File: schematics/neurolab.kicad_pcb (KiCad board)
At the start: 2 copper layers, 127 x 53.6 mm, 159 parts, among them J1 GS3, J10 GS3, J12 GS3, J13 GS3, J14 GS3, J15 GS3, J16 Channel, J17 External, J18 USB_OTG, J19 GS3, J2 GS3, J24 GS2, J3 GS3, J32 Bluetooth, J33 Reset Select, J34 GS2, J4 GS2, J5 GS2, J6 GS3, J7 GS3, J8 PowerOut, J9 GS3, Q1 2N7002, U1 ADP1720ARMZ-5, U10 OPA2111KP, U11 AD8422ARMZ, U12 OP4117, U13 OPA2111KP, U14 AD8422ARMZ, U15 OP4117, U16 AD7173, U17 ADR445BR, U18 Arduino, U2 ADP1720ARMZ-3.3, U3 AD8475, U4 AD8475, U5 MAX7480ESA+, U6 MAX7480ESA+, U7 MAX7480ESA+, U8 MAX7480ESA+, U9 TLC555CD, Y1 FA-20H

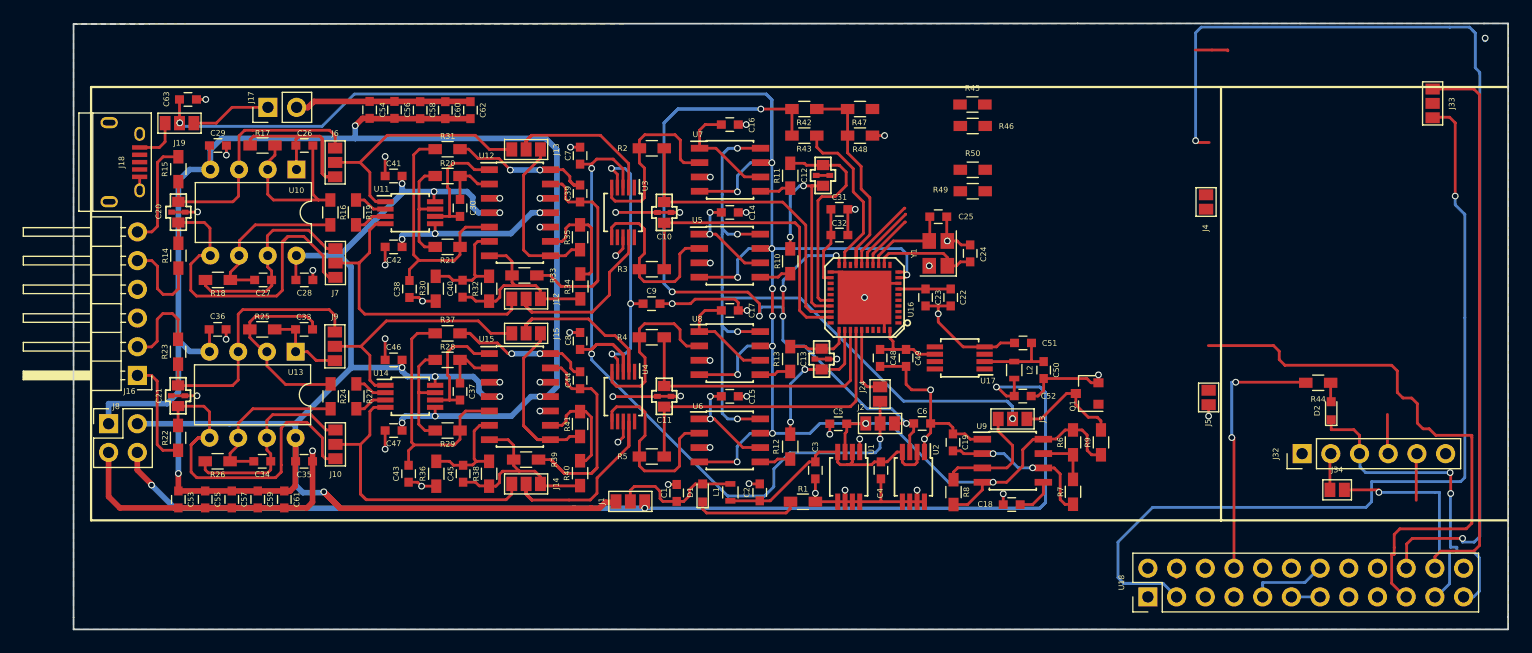
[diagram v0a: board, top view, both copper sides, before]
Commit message: optimize: final routing
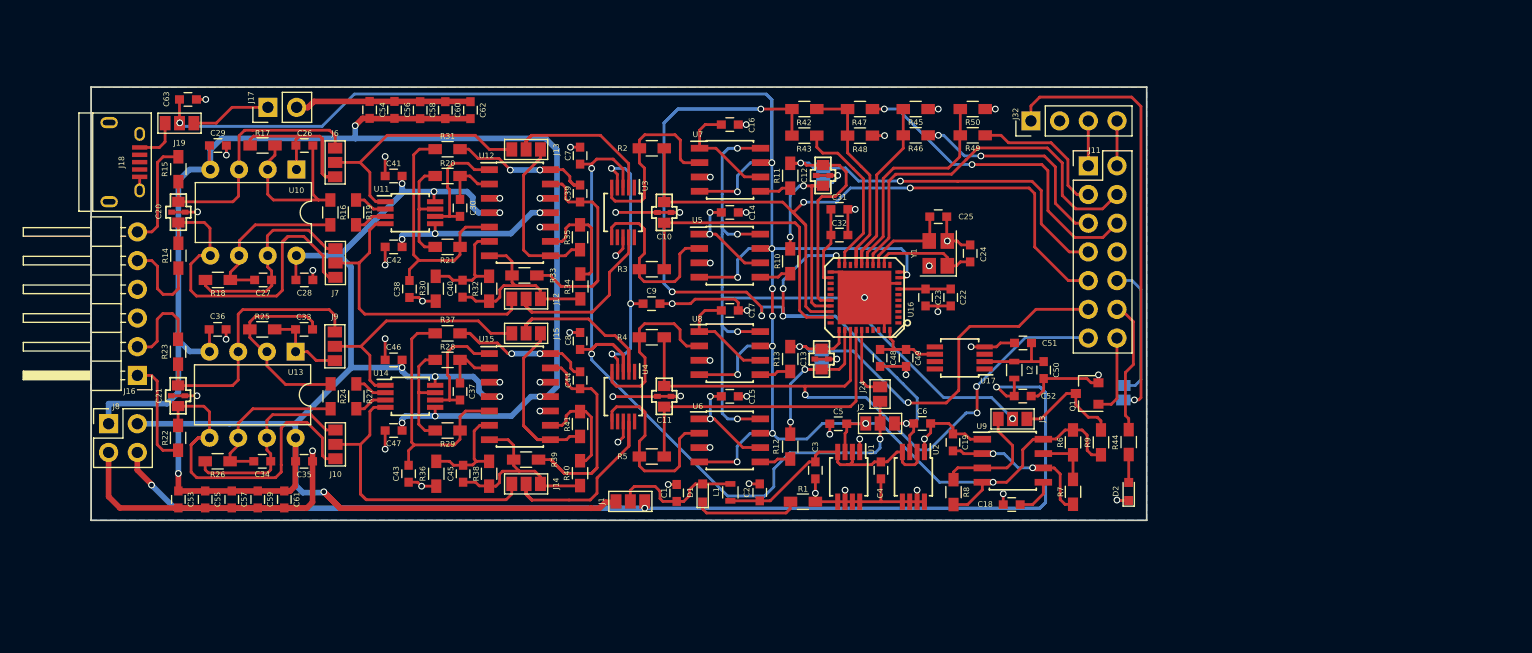
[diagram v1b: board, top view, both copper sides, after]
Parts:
- removed J33: Reset Select, Connectors:GS3
- removed U18: Arduino, Pin_Headers:Pin_Header_Straight_2x12_Pitch2.54mm
- added J11: ProMini, Pin_Headers:Pin_Header_Straight_2x07_Pitch2.54mm, F.Cu at (179.8, 84.8)
- J32: footprint Pin_Headers:Pin_Header_Straight_1x06_Pitch2.54mm -> Pin_Headers:Pin_Header_Straight_1x04_Pitch2.54mm
- J34, J4, J5: moved to B.Cu
- moved J32 38.0 mm to (174.8, 80.9)
- moved J5 34.4 mm to (156.2, 101.9), turned to 0 degrees
- moved J4 34.0 mm to (156.4, 85.7), turned to 0 degrees
- moved J34 20.8 mm to (183.0, 104.9), turned to 0 degrees
- moved D2 19.3 mm to (183.4, 113.7)
- moved R44 17.6 mm to (183.4, 109.3), turned to 270 degrees
- moved R50 5.38 mm to (169.6, 79.8)
- moved R46 5.12 mm to (164.6, 82.2)
- moved R45 5.04 mm to (164.6, 79.8)
- moved R49 4.95 mm to (169.6, 82.2)
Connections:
- J32 pad 1: (no net) -> VCC
- J32 pad 2: VCC -> GND
- J32 pad 3: GND -> TxO
- J32 pad 4: TxO -> RxI
- R44 pad 1: Net-(D2-Pad2) -> Net-(J11-Pad12)
- R44 pad 2: Net-(R44-Pad2) -> Net-(D2-Pad2)
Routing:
- net Net-(J33-Pad1): track 80.7 -> 0.00 mm, vias 1 -> 0
- net AD3: track 110.3 -> 50.9 mm
- net Net-(J33-Pad3): track 49.6 -> 0.00 mm
- net GND: track 225.7 -> 186.9 mm, vias 57 -> 58
- net VCC: track 3.28 -> 39.2 mm, vias 0 -> 1
- net AD1: track 27.7 -> 62.5 mm, vias 0 -> 2
- net AD0: track 25.5 -> 59.0 mm, vias 0 -> 3
- net MOSI: track 5.02 -> 33.9 mm
- net CS: track 2.54 -> 29.0 mm, vias 0 -> 2
- net Net-(R44-Pad2): track 23.3 -> 0.00 mm, vias 2 -> 0
- net SCL: track 0.00 -> 19.6 mm, vias 0 -> 2
- net AD2: track 56.5 -> 40.5 mm, vias 0 -> 2
- net /ADConverter/DI: track 5.90 -> 20.1 mm
- net /ADConverter/SCL: track 6.64 -> 19.7 mm
- net Net-(J11-Pad12): track 0.00 -> 11.9 mm
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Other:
- board size 127 x 53.6 mm -> 93.4 x 38.3 mm
